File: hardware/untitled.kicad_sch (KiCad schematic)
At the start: 27 parts, among them U1 F1C100s

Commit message: Board design started
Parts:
- U1: footprint 3340:QFN-88_EP_10x10_Pitch0.4mm -> Package_DFN_QFN:ArtInChip_QFN-88-1EP_10x10mm_P0.4mm_EP6.74x6.74mm
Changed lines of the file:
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@@
 			)
 		)
-		(property "Footprint" "3340:QFN-88_EP_10x10_Pitch0.4mm"
+		(property "Footprint" "Package_DFN_QFN:ArtInChip_QFN-88-1EP_10x10mm_P0.4mm_EP6.74x6.74mm"
 			(at 43.18 49.53 0)
 			(effects
@@
 			)
 		)
-		(property "Footprint" "3340:QFN-88_EP_10x10_Pitch0.4mm"
+		(property "Footprint" "Package_DFN_QFN:ArtInChip_QFN-88-1EP_10x10mm_P0.4mm_EP6.74x6.74mm"
 			(at 173.99 38.1 0)
 			(effects

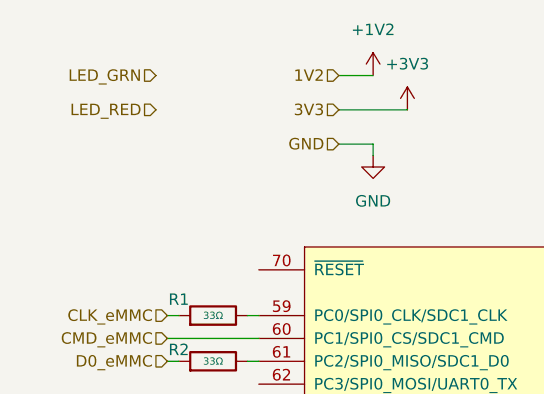
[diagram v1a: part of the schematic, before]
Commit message: PCB major changes
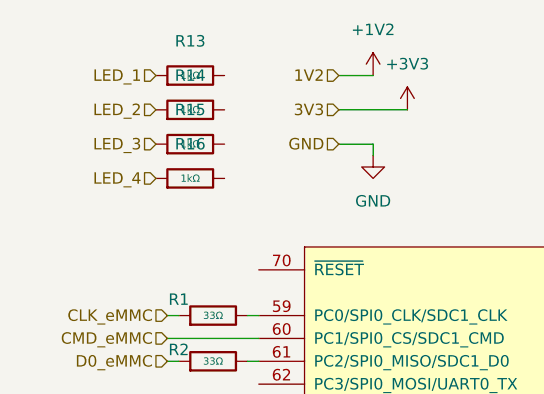
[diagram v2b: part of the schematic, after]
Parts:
- added R13, R14, R15, R16: 1kΩ, PCM_JLCPCB:R_0603, symbol PCM_JLCPCB-Resistors:0603,1kΩ
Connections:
- new net LED_1: R13.1
- new net LED_2: R14.1
- new net LED_3: R15.1
- new net LED_4: R16.1
